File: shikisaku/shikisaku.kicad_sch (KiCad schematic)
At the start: 22 parts, among them Q1 2SC1815, Q2 2SC1815, Q3 2SC1815, SW1 SW_Reset, SW2 SW_Push, SW3 SW_SPST, U1 ProMicro, U2 MMC5603, U3 HC-SR04, U4 HC-SR04, U5 XCL103

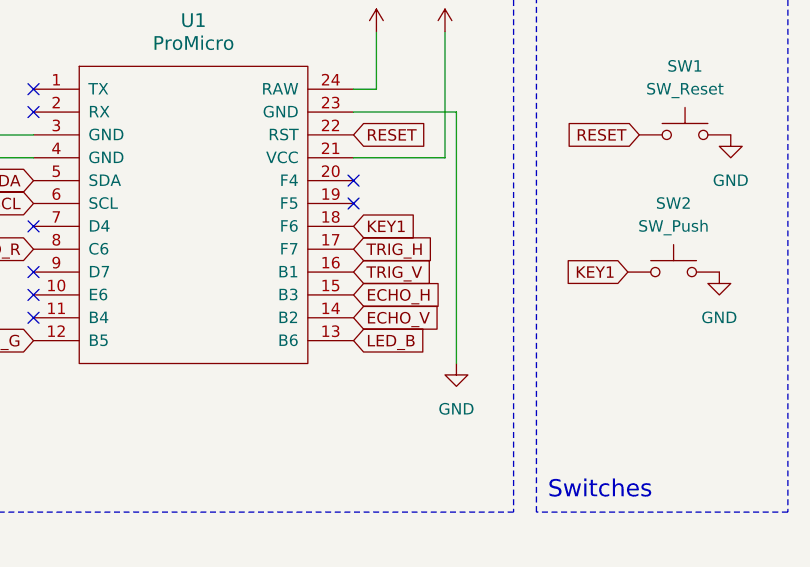
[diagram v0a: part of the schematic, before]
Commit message: layout footprints
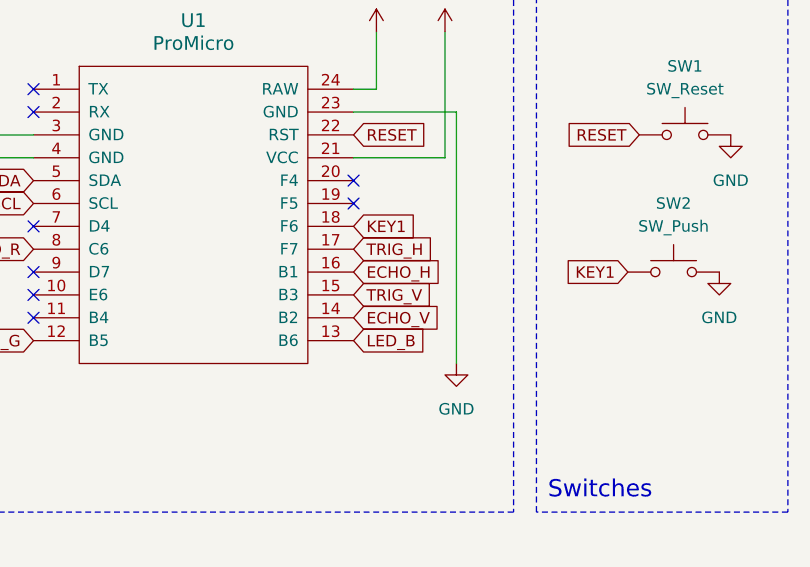
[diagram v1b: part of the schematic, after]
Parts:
- BT1: footprint Connector_JST:JST_XH_B2B-XH-A_1x02_P2.50mm_Vertical -> Connector_JST:JST_XH_S2B-XH-A_1x02_P2.50mm_Horizontal
- U1: footprint promicro:ProMicro -> promicro:ProMicro-EnforcedTop
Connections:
- net ECHO_H: now also U1.16 (B1); no longer U1.15 (B3)
- net TRIG_V: now also U1.15 (B3); no longer U1.16 (B1)
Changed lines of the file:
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@@
     )
   )
-  (global_label "ECHO_H" (shape input) (at 81.28 116.84 0) (fields_autoplaced)
+  (global_label "ECHO_H" (shape input) (at 81.28 114.3 0) (fields_autoplaced)
     (effects (font (size 1.27 1.27)) (justify left))
-    (property "Intersheetrefs" "${INTERSHEET_REFS}" (at 91.6433 116.84 0)
+    (property "Intersheetrefs" "${INTERSHEET_REFS}" (at 91.6433 114.3 0)
       (effects (font (size 1.27 1.27)) (justify left) hide)
     )
@@
     )
   )
-  (global_label "TRIG_V" (shape input) (at 81.28 114.3 0) (fields_autoplaced)
+  (global_label "TRIG_V" (shape input) (at 81.28 116.84 0) (fields_autoplaced)
     (effects (font (size 1.27 1.27)) (justify left))
-    (property "Intersheetrefs" "${INTERSHEET_REFS}" (at 90.4338 114.3 0)
+    (property "Intersheetrefs" "${INTERSHEET_REFS}" (at 90.4338 116.84 0)
       (effects (font (size 1.27 1.27)) (justify left) hide)
     )
@@
       (effects (font (size 1.524 1.524)))
     )
-    (property "Footprint" "promicro:ProMicro" (at 66.04 139.7 0)
+    (property "Footprint" "promicro:ProMicro-EnforcedTop" (at 66.04 139.7 0)
       (effects (font (size 1.524 1.524)) hide)
     )
@@
       (effects (font (size 1.27 1.27)) (justify left))
     )
-    (property "Footprint" "Connector_JST:JST_XH_B2B-XH-A_1x02_P2.50mm_Vertical" (at 59.69 55.626 90)
-      (effects (font (size 1.27 1.27)) hide)
-    )
+    (property "Footprint" "Connector_JST:JST_XH_S2B-XH-A_1x02_P2.50mm_Horizontal" (at 59.69 55.626 90)
+      (effects (font (size 1.27 1.27)) hide)
+    )
